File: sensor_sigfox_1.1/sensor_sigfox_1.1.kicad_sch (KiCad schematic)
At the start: 36 parts, among them IC1 AS5600-ASOM, IC2 WSSFM11R2DAT, J1 UDPI, J2 Battery, J4 Conn_Coaxial, Q1 DMC2053UVT, U1 MLX90393, U2 ATtiny826-X, U3 MT3608, Y1 Crystal

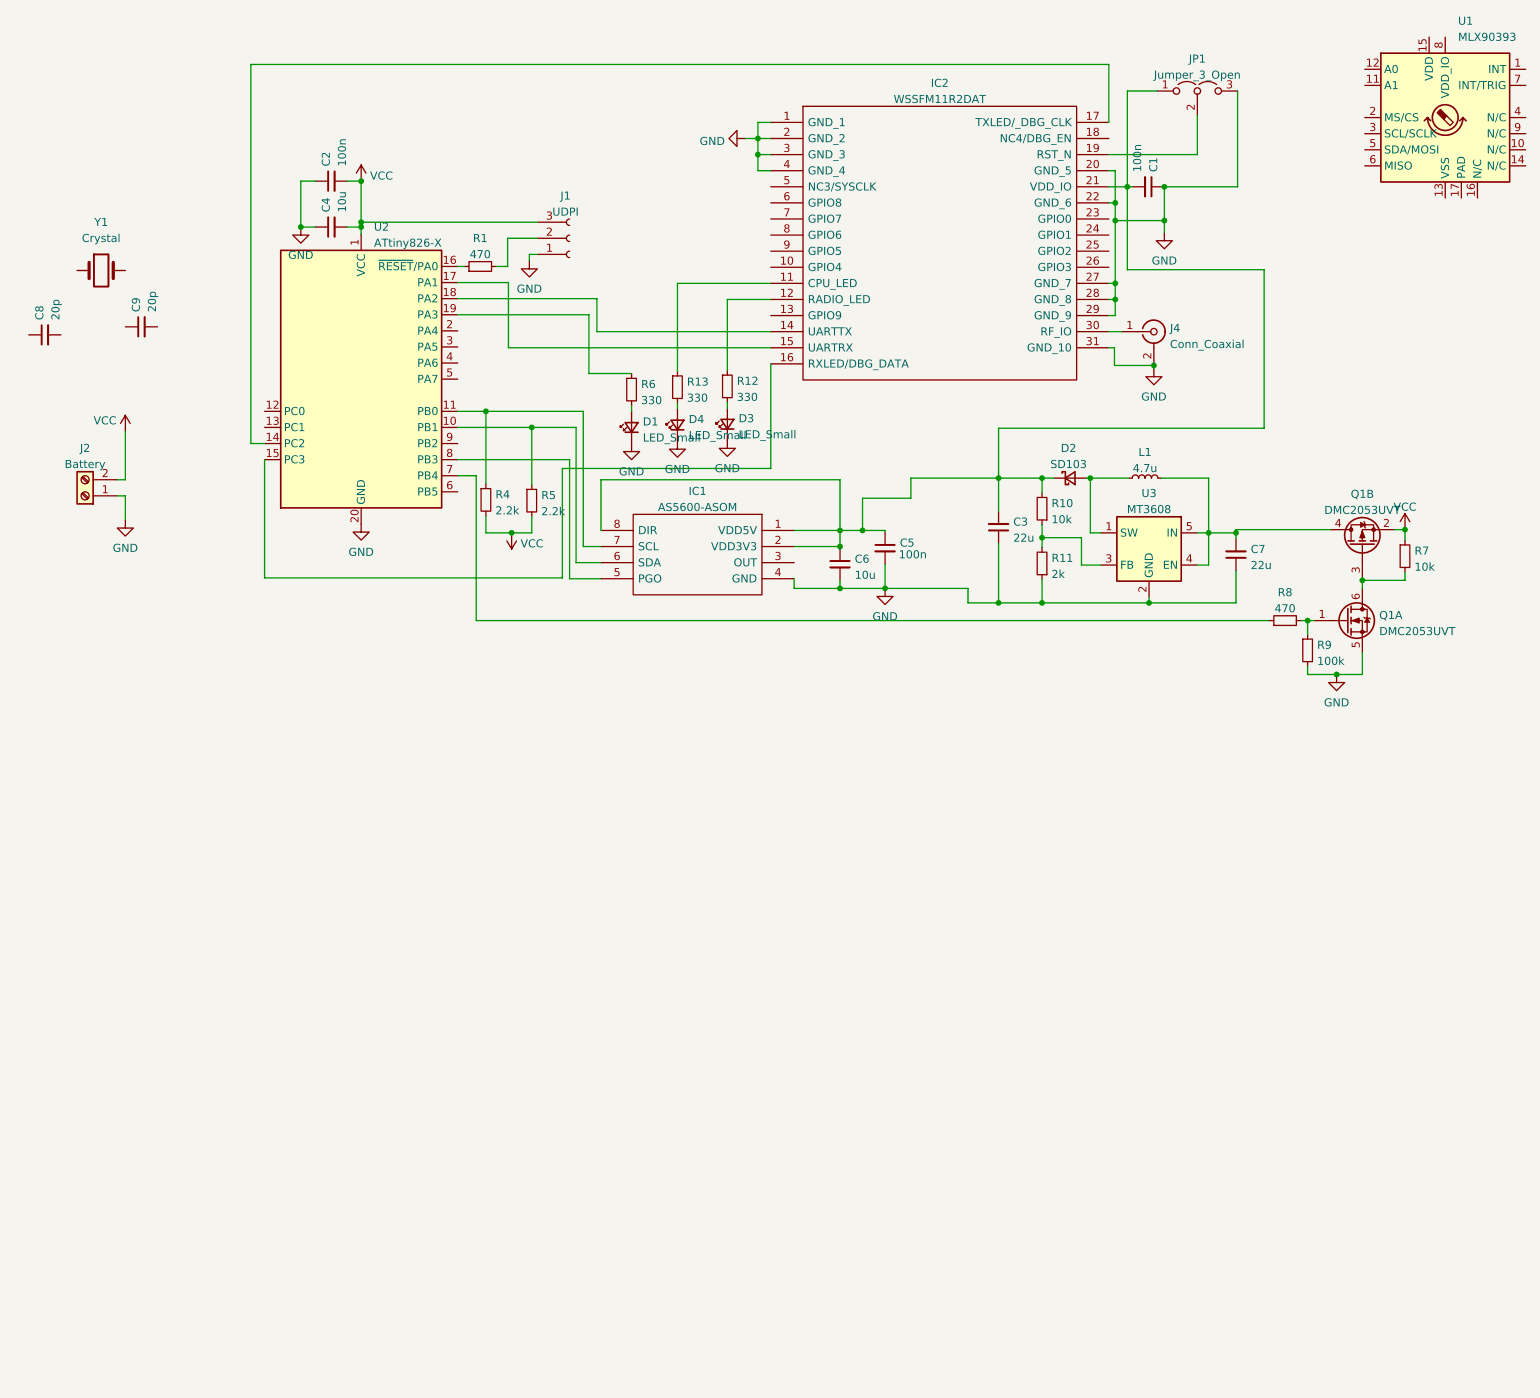
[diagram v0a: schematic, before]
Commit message: iniciar conexiones a nuevos comps
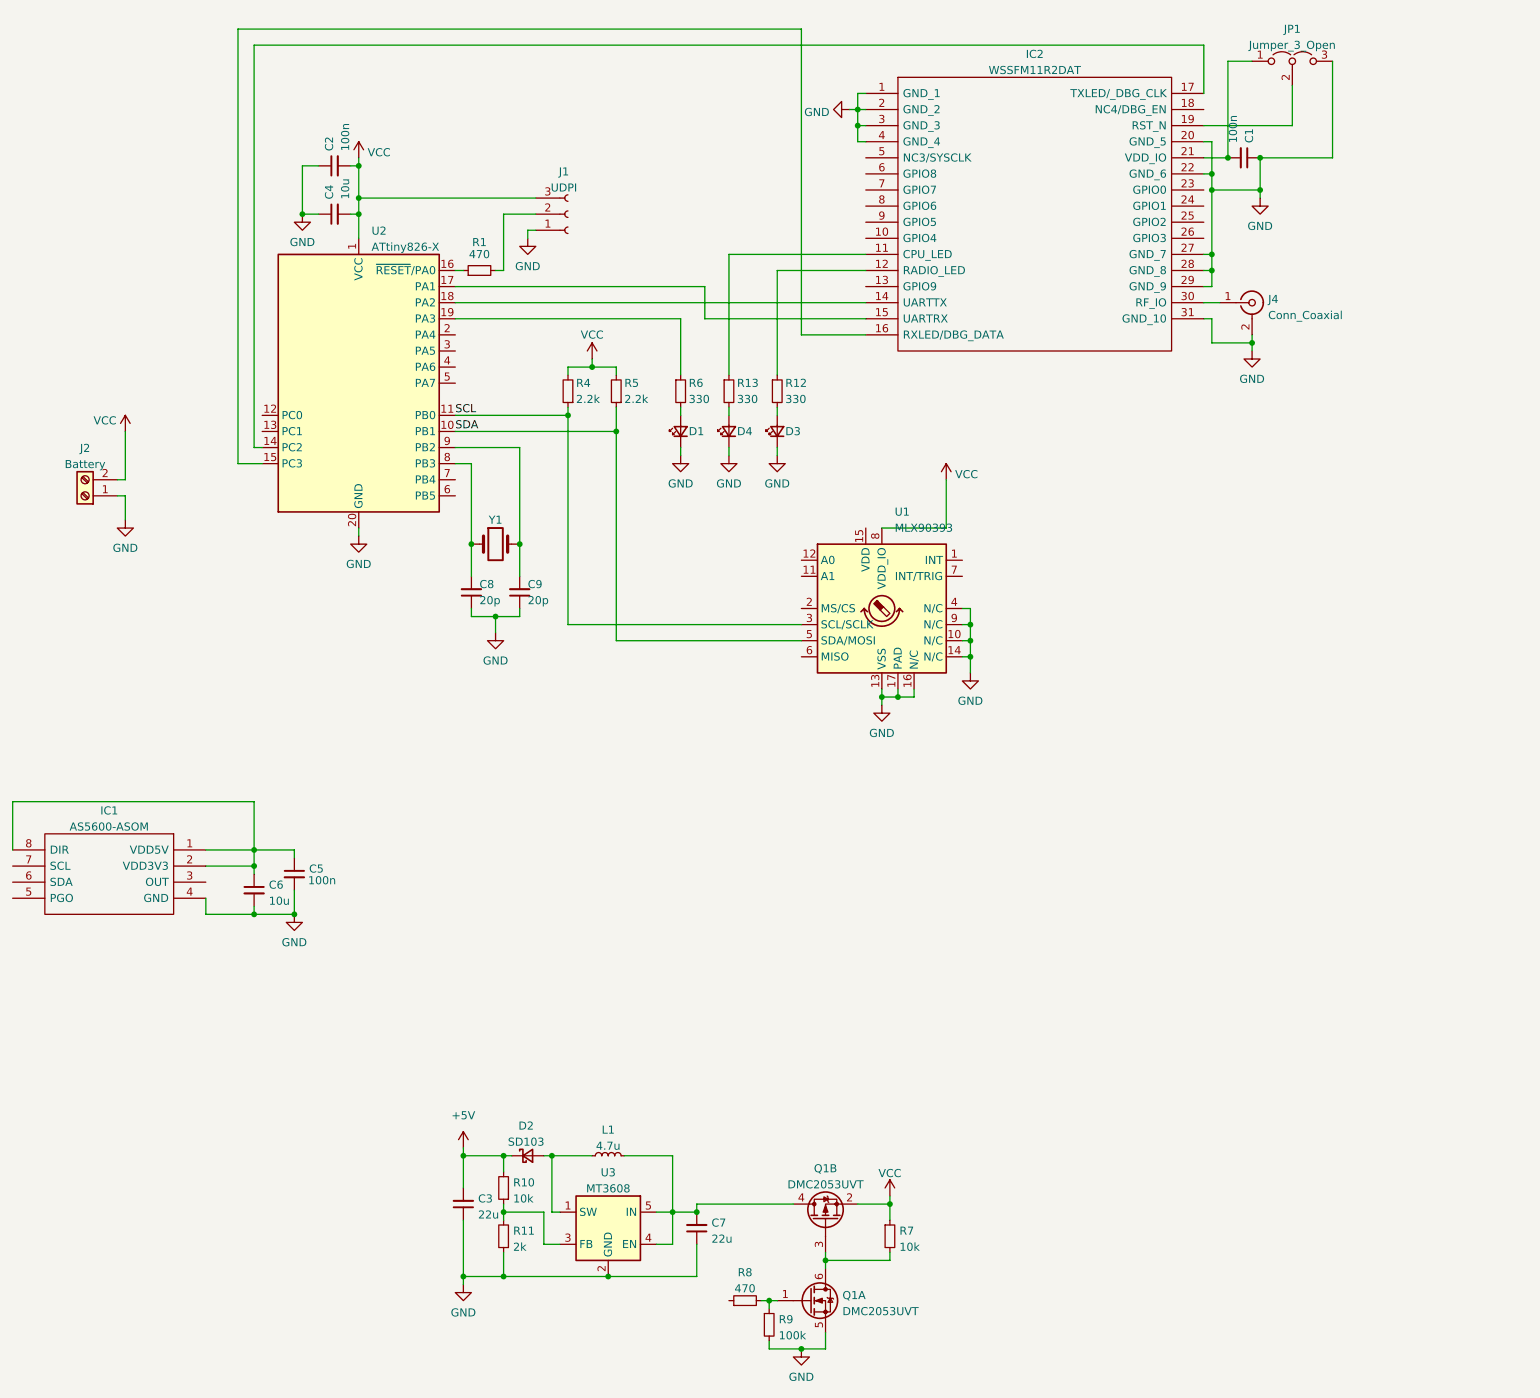
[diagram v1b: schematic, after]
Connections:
- net GND: now also C8.1, C9.1, U1.10 (N/C), U1.13 (VSS), U1.14 (N/C), U1.16 (N/C), U1.17 (PAD), U1.4 (N/C), U1.9 (N/C)
- net VCC: now also U1.8 (VDD_IO)
- net SDA: now reaches R5.1, U2.10 (PB1)
- net SDA: now also U1.5 (SDA/MOSI); no longer IC1.6 (SDA)
- net SCL: now reaches R4.1, U2.11 (PB0)
- net SCL: now also U1.3 (SCL/SCLK); no longer IC1.7 (SCL)
- net at U2.7 (PB4): no longer R8.1
- net at U2.8 (PB3): now also C8.2, Y1.1; no longer IC1.5 (PGO)
- net at U2.9 (PB2): now also C9.2, Y1.2
- new net: C1.2, IC2.21 (VDD_IO), JP1.1 (A)
- new net: C5.1, C6.1, IC1.1 (VDD5V), IC1.2 (VDD3V3), IC1.8 (DIR)
- new net +5V: C3.2, D2.1 (K), R10.2
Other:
- moved on the sheet: C1, C2, C3, C4, C5, C6, C7, C8, C9, D1, D2, D3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
